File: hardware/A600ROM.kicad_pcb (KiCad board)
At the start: 4 copper layers, 106.7 x 39.4 mm, 11 parts, among them J1 Conn_01x02_Pin, J2 Conn_01x02_Pin, U1 Kickstart A600 ROM, U2 M29F160F

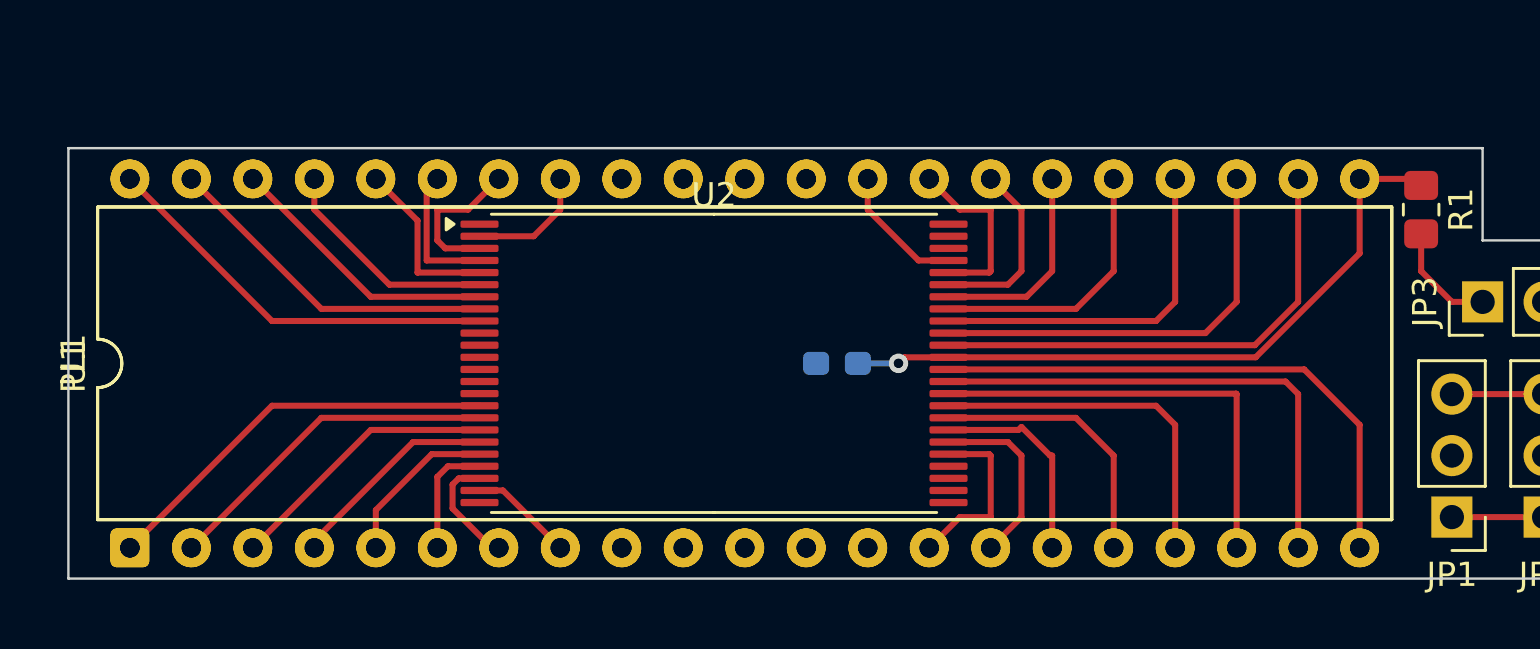
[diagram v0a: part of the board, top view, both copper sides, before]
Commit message: Add connectors
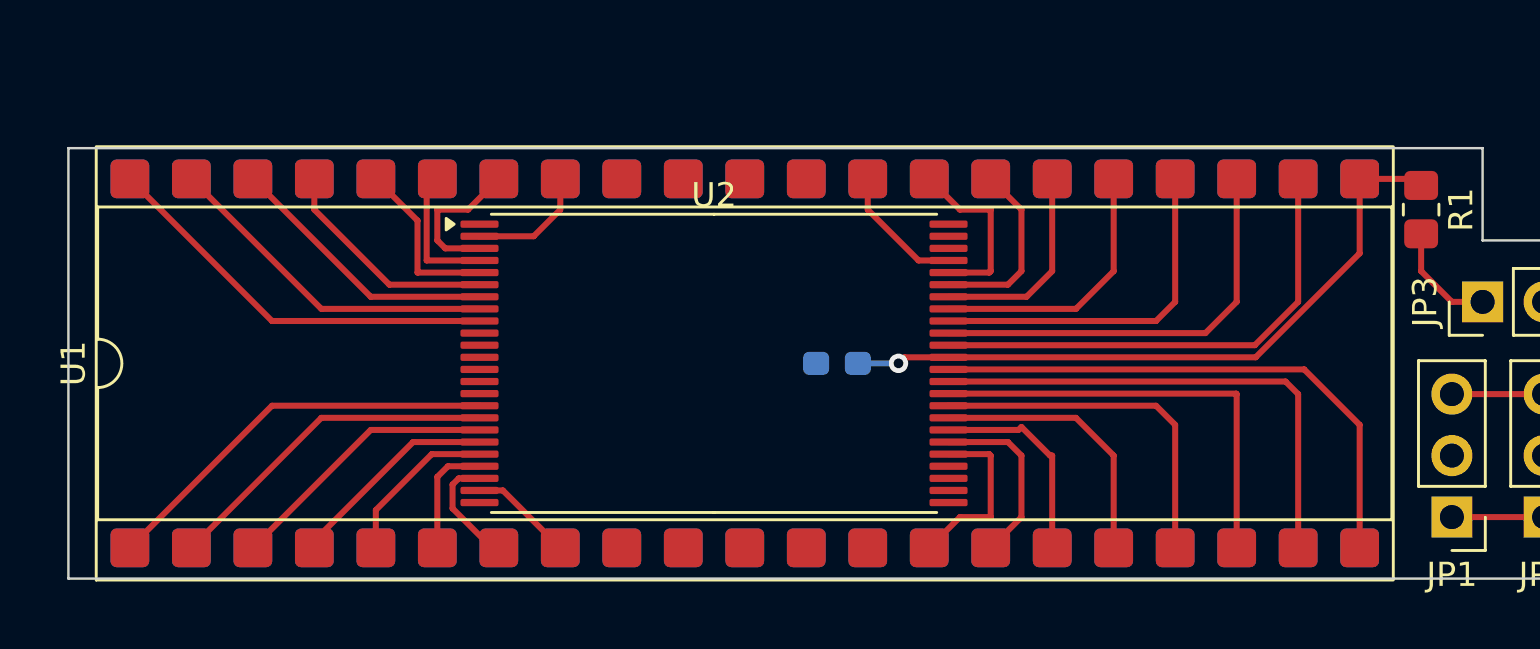
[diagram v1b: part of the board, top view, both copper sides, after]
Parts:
- PL1: footprint Package_DIP:DIP-42_W15.24mm -> A600ROM:DIP-42_W15.24mm_SMDHeader_SmallPads; moved to B.Cu
- U1: footprint Package_DIP:DIP-42_W15.24mm -> A600ROM:DIP-42_W15.24mm_SMDSocket_SmallPads
- moved PL1 26.5 mm to (122.9, 99.5), turned to -90 degrees
- moved U1 26.5 mm to (122.9, 99.5)
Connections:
- net /~{U6_ROMEN} renamed /~{U6_CS}
- J1 pad 2: /~{FLASH} -> /~{FLASH}_GAYLE
- J2 pad 2: /~{FLASH} -> /~{FLASH}_GAYLE
- JP1 pad 3: /~{FLASH} -> /~{U5_FLASH}
- SK1 pad 11: /~{FLASH} -> /~{FLASH}_GAYLE
